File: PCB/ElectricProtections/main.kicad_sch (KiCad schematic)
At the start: 3 parts

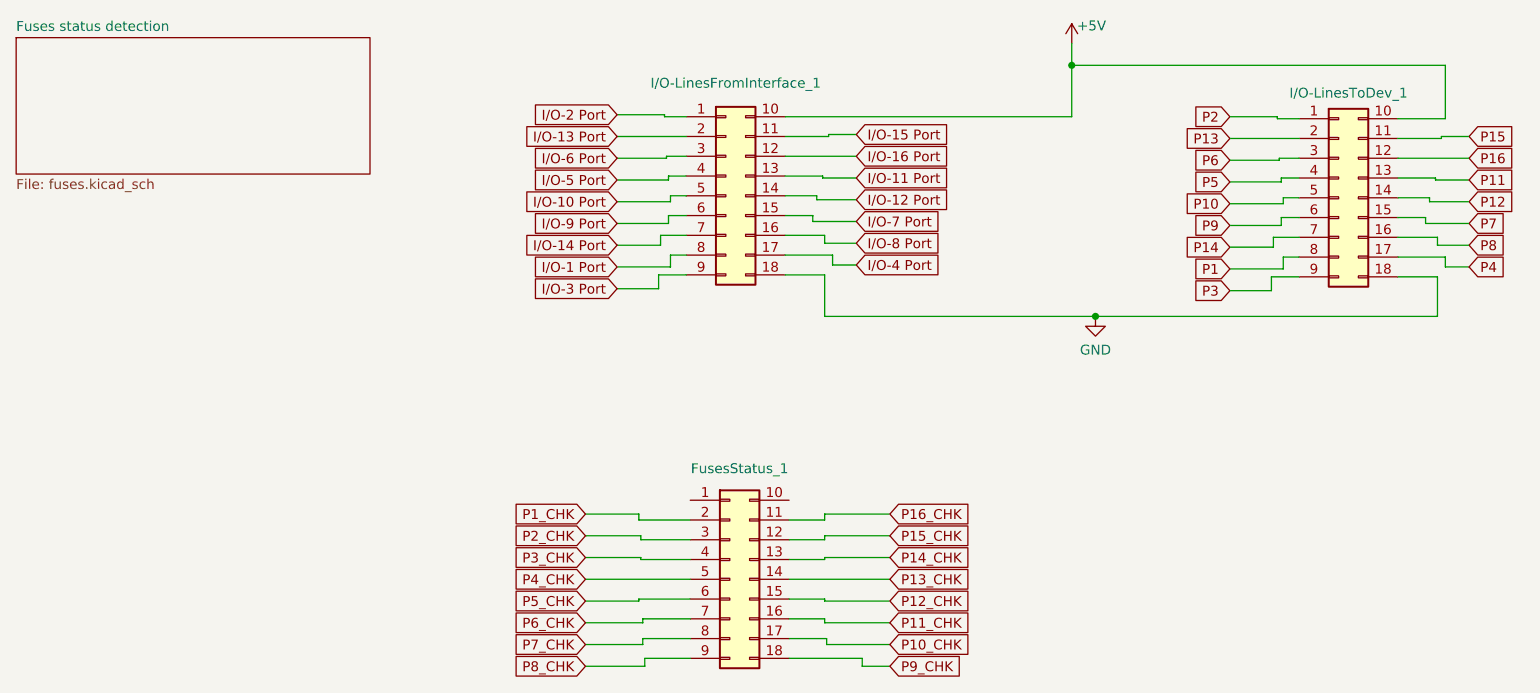
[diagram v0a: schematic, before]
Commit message: Updates
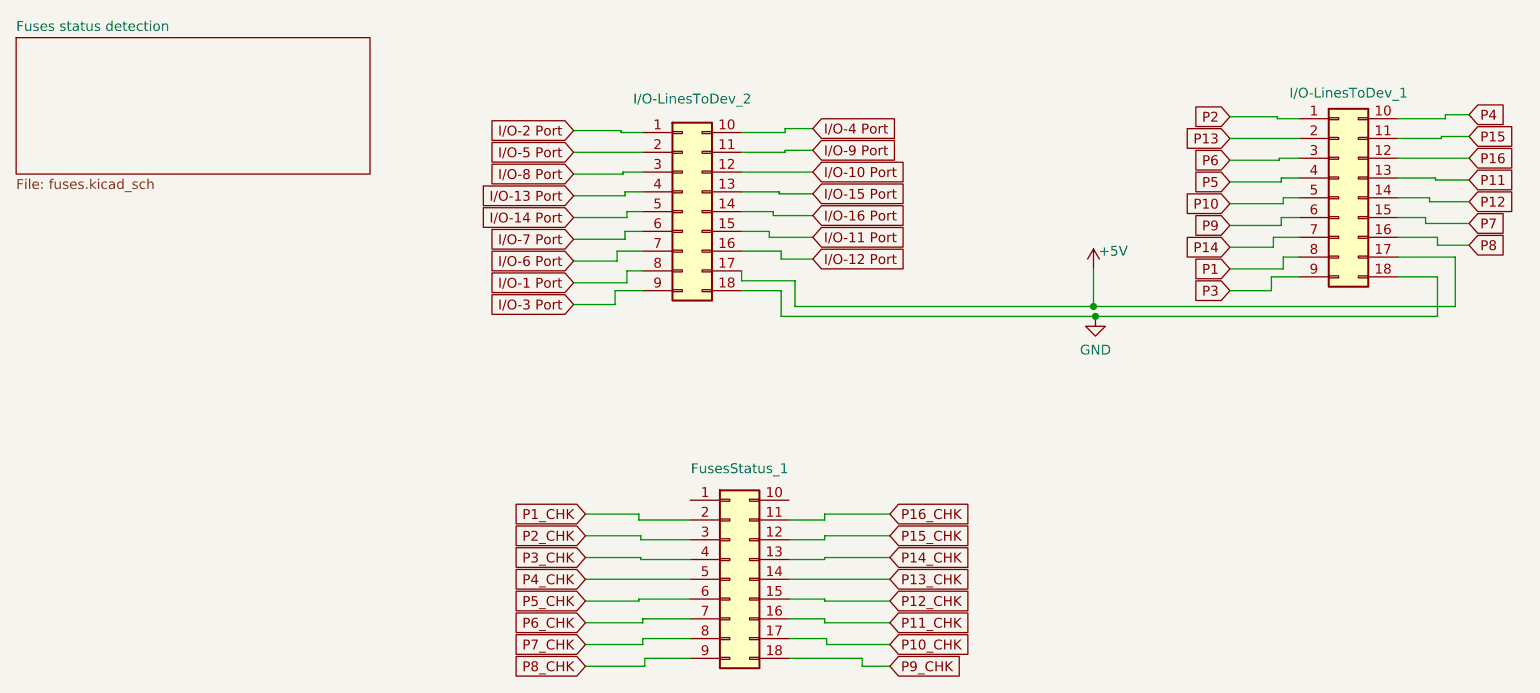
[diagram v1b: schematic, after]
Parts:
- removed I/O-LinesFromInterface_1: Conn_02x09_Top_Bottom, Connector_PinHeader_2.54mm:PinHeader_2x09_P2.54mm_Vertical, symbol Connector_Generic:Conn_02x09_Top_Bottom
- added I/O-LinesToDev_2: Conn_02x09_Top_Bottom, Connector_PinHeader_2.54mm:PinHeader_2x09_P2.54mm_Vertical, symbol Connector_Generic:Conn_02x09_Top_Bottom
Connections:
- net +5V: now also I/O-LinesToDev_1.17 (Pin_17), I/O-LinesToDev_2.17 (Pin_17); no longer I/O-LinesToDev_1.10 (Pin_10)
- net GND: now also I/O-LinesToDev_2.18 (Pin_18)
- net I/O-1 Port: now also I/O-LinesToDev_2.8 (Pin_8)
- net I/O-10 Port: now also I/O-LinesToDev_2.12 (Pin_12)
- net I/O-11 Port: now also I/O-LinesToDev_2.15 (Pin_15)
- net I/O-12 Port: now also I/O-LinesToDev_2.16 (Pin_16)
- net I/O-13 Port: now also I/O-LinesToDev_2.4 (Pin_4)
- net I/O-14 Port: now also I/O-LinesToDev_2.5 (Pin_5)
- net I/O-15 Port: now also I/O-LinesToDev_2.13 (Pin_13)
- net I/O-16 Port: now also I/O-LinesToDev_2.14 (Pin_14)
- net I/O-2 Port: now also I/O-LinesToDev_2.1 (Pin_1)
- net I/O-3 Port: now also I/O-LinesToDev_2.9 (Pin_9)
- net I/O-4 Port: now also I/O-LinesToDev_2.10 (Pin_10)
- net I/O-5 Port: now also I/O-LinesToDev_2.2 (Pin_2)
- net I/O-6 Port: now also I/O-LinesToDev_2.7 (Pin_7)
- net I/O-7 Port: now also I/O-LinesToDev_2.6 (Pin_6)
- net I/O-8 Port: now also I/O-LinesToDev_2.3 (Pin_3)
- net I/O-9 Port: now also I/O-LinesToDev_2.11 (Pin_11)
- net P4: now also I/O-LinesToDev_1.10 (Pin_10); no longer I/O-LinesToDev_1.17 (Pin_17)
